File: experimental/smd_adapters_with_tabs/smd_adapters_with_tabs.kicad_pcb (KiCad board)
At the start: 2 copper layers, 79.8 x 64.6 mm, 34 parts

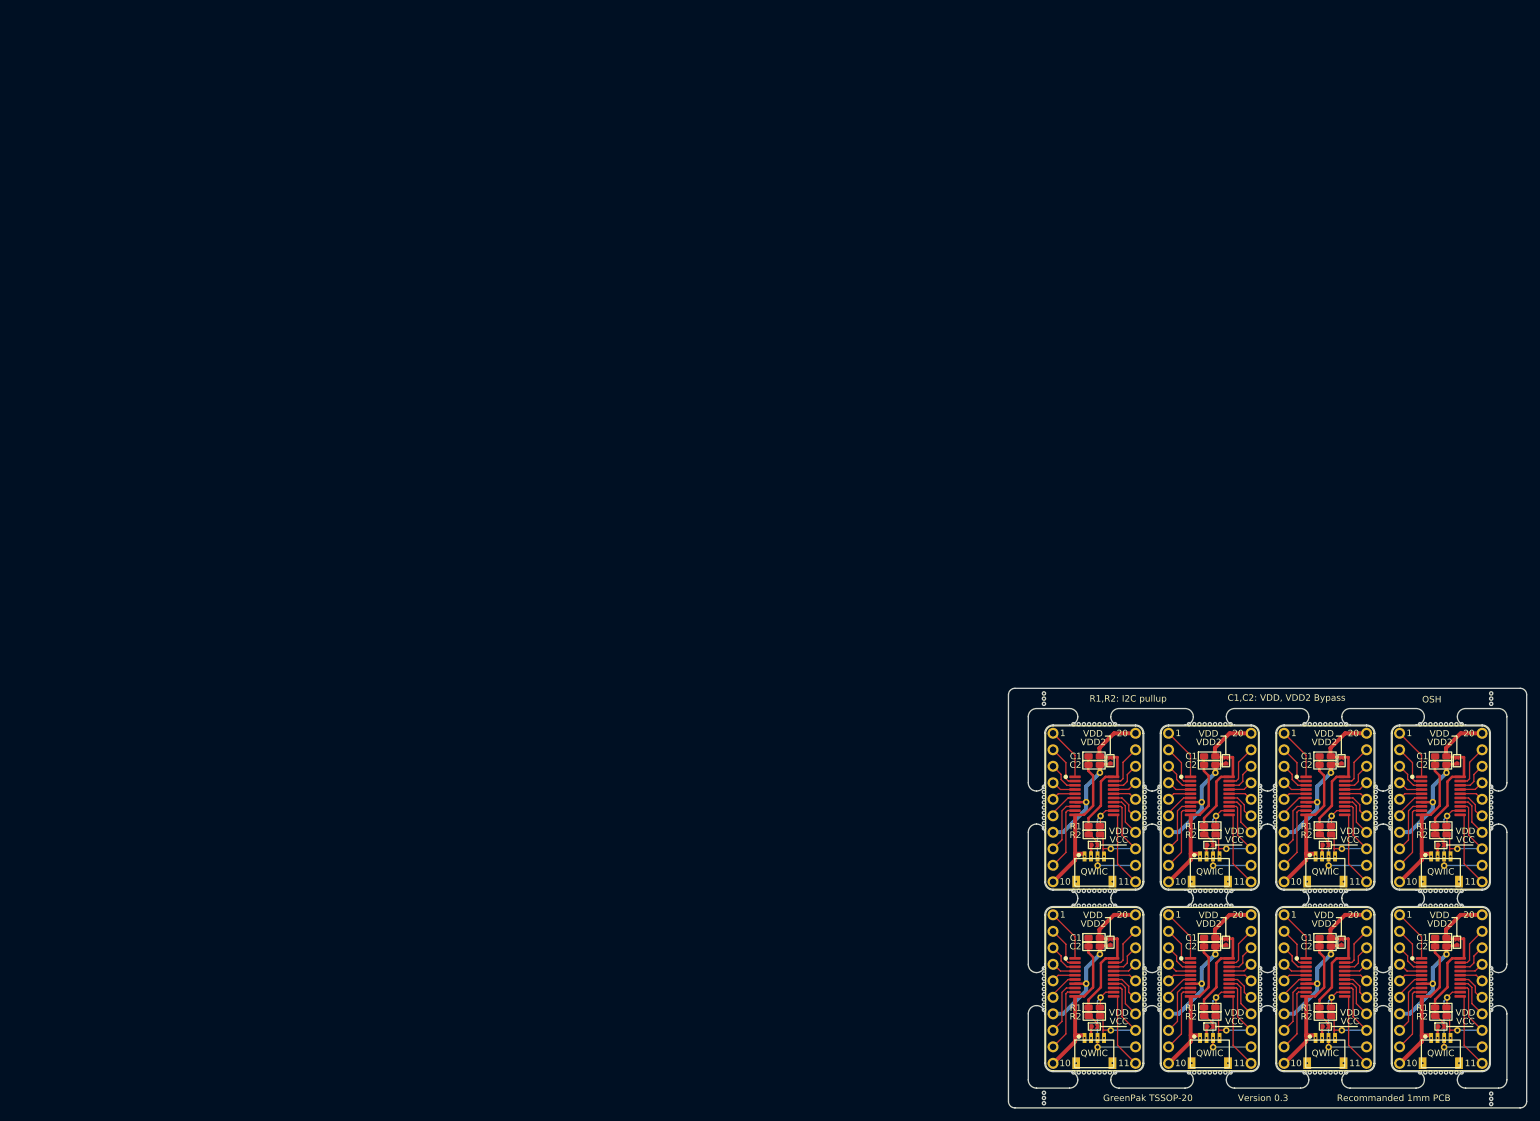
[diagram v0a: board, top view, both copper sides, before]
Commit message: Updated gerber.
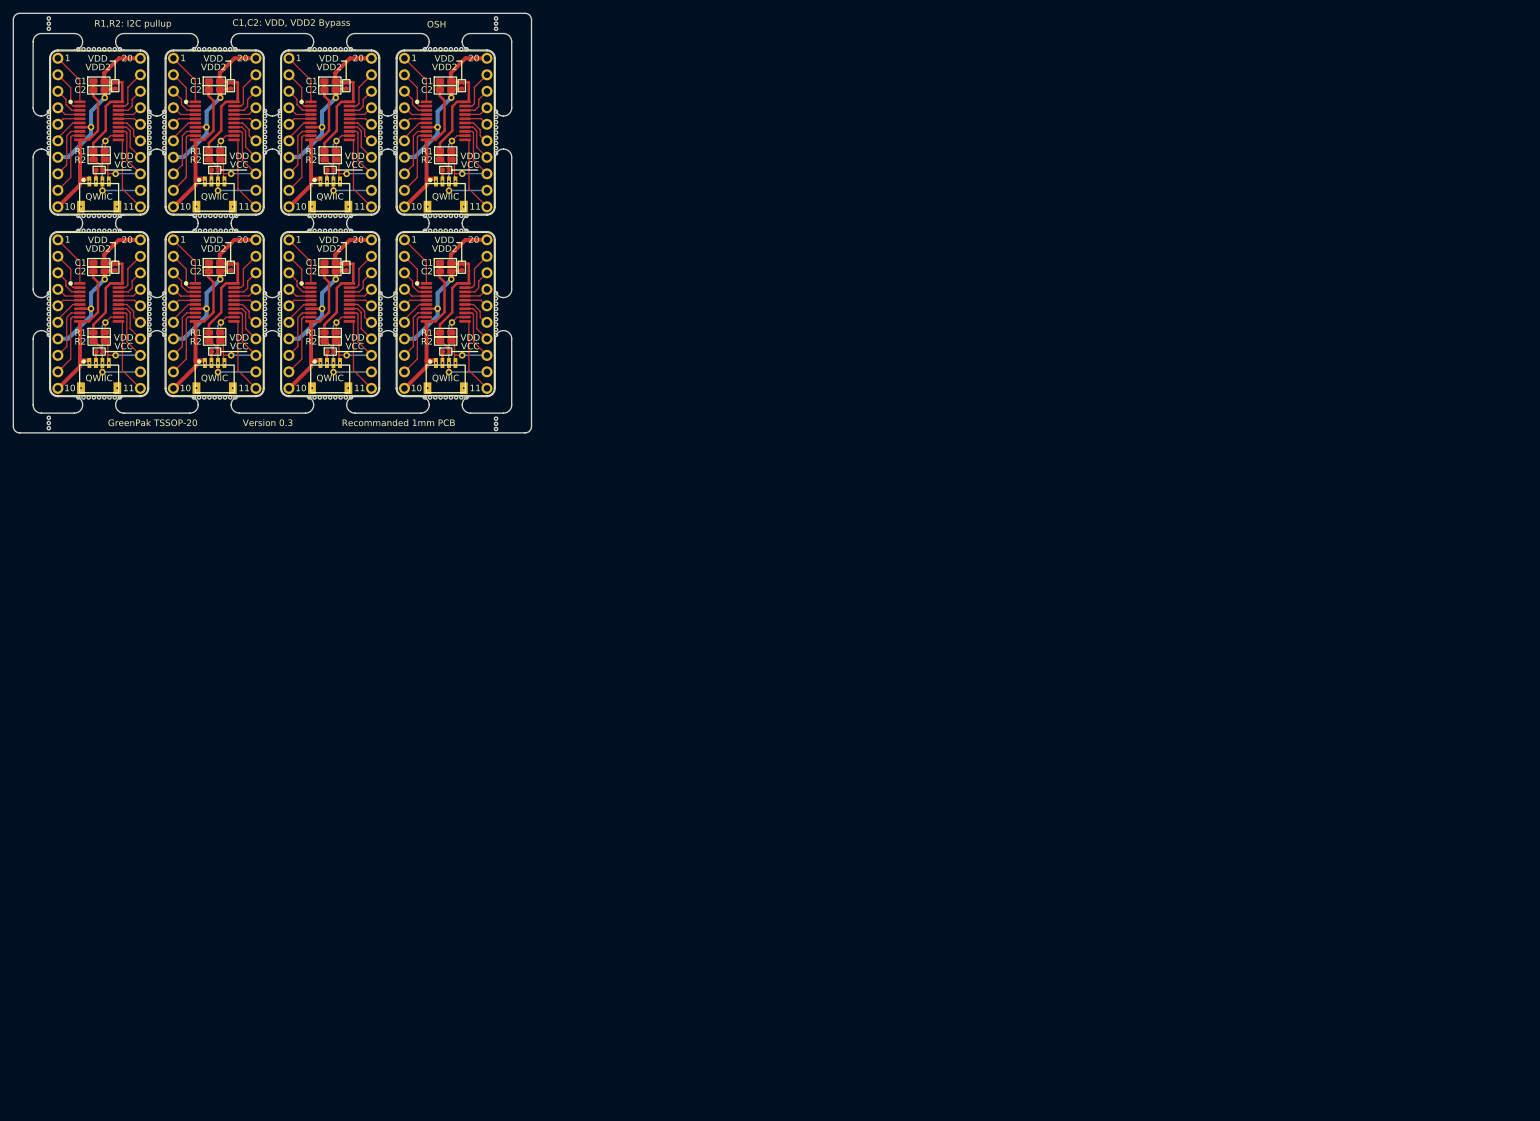
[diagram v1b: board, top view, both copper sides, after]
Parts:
- moved mouse-bite-2.54mm-slot 185.1 mm to (38.9, 23.7)
- moved mouse-bite-2.54mm-slot 185.1 mm to (3.30, -21.2)
- moved REF** 185.1 mm to (30.0, 6.86)
- moved REF** 185.1 mm to (-5.59, -21.1)
- moved REF** 185.1 mm to (-5.59, 6.86)
- moved REF** 185.1 mm to (30.0, -21.1)
- moved REF** 185.1 mm to (12.2, -21.1)
- moved REF** 185.1 mm to (-23.4, -21.1)
- moved REF** 185.1 mm to (-23.4, 6.86)
- moved REF** 185.1 mm to (12.2, 6.86)
- moved mouse-bite-2.54mm-slot 185.1 mm to (30.0, -7.11)
- moved mouse-bite-2.54mm-slot 185.1 mm to (-14.5, -21.1)
- moved mouse-bite-2.54mm-slot 185.1 mm to (38.9, -37.8)
- moved mouse-bite-2.54mm-slot 185.1 mm to (-5.59, 20.8)
- moved mouse-bite-2.54mm-slot 185.1 mm to (-32.3, 23.6)
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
